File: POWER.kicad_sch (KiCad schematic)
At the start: 42 parts, among them IC1 MP2491CGQB-P, J1 Jack-DC, U1 5V-DCDC, U2 3v3-DCDC, U5 TPS55340RTER

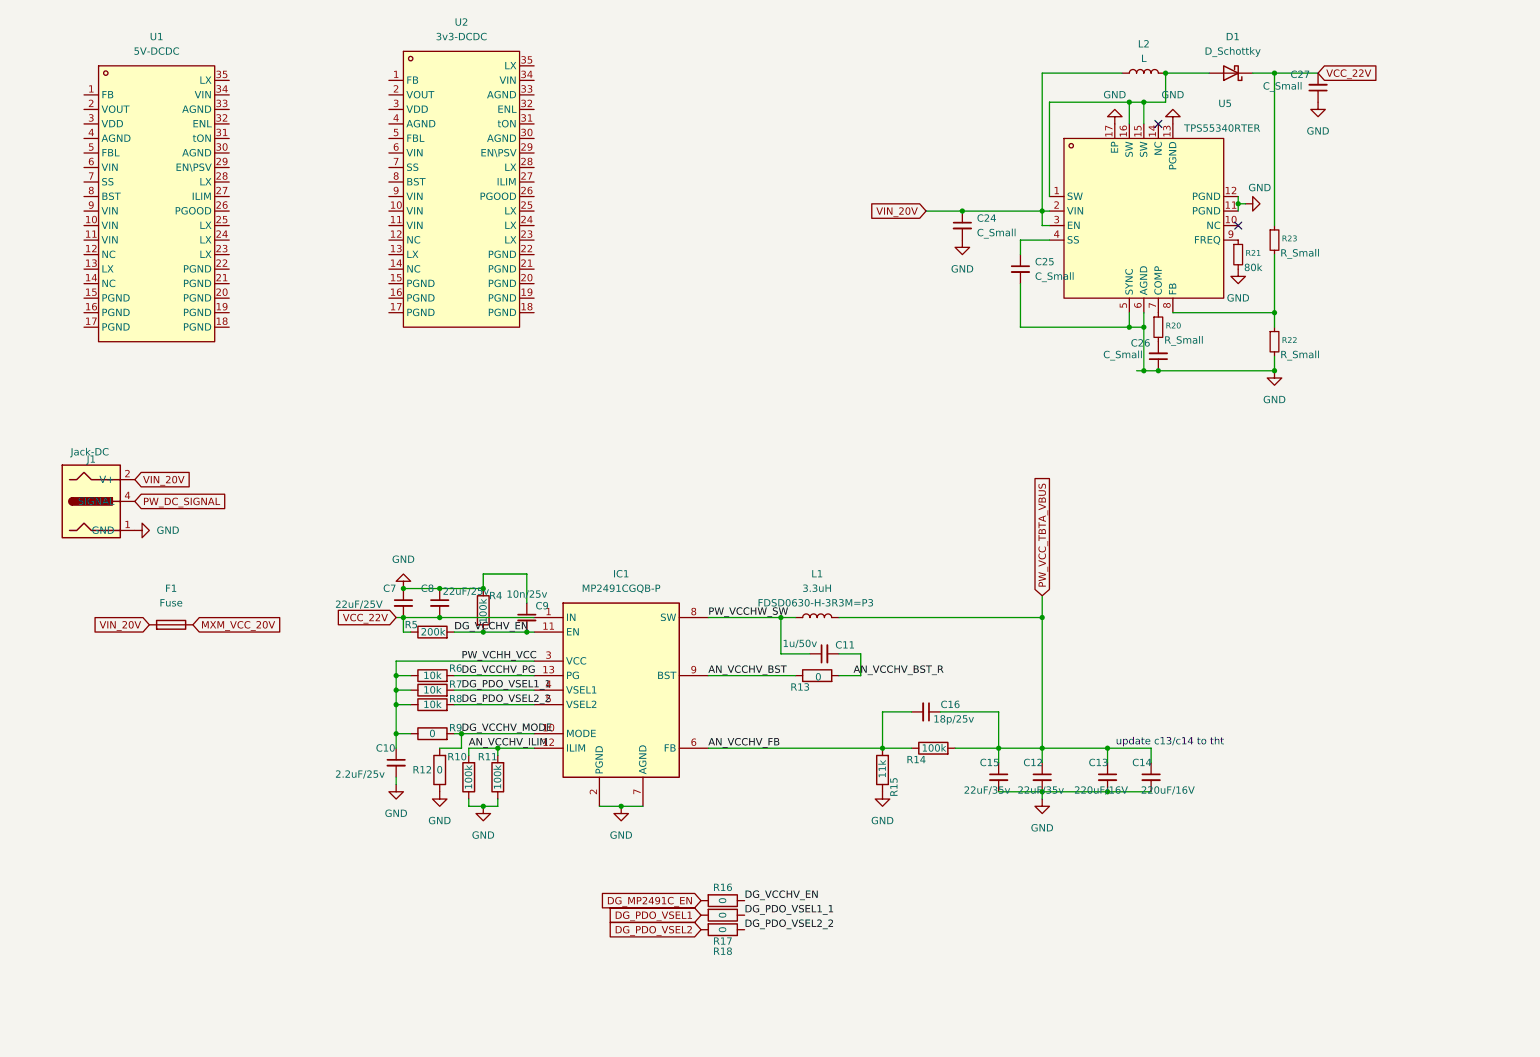
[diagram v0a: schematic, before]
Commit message: update readme.md
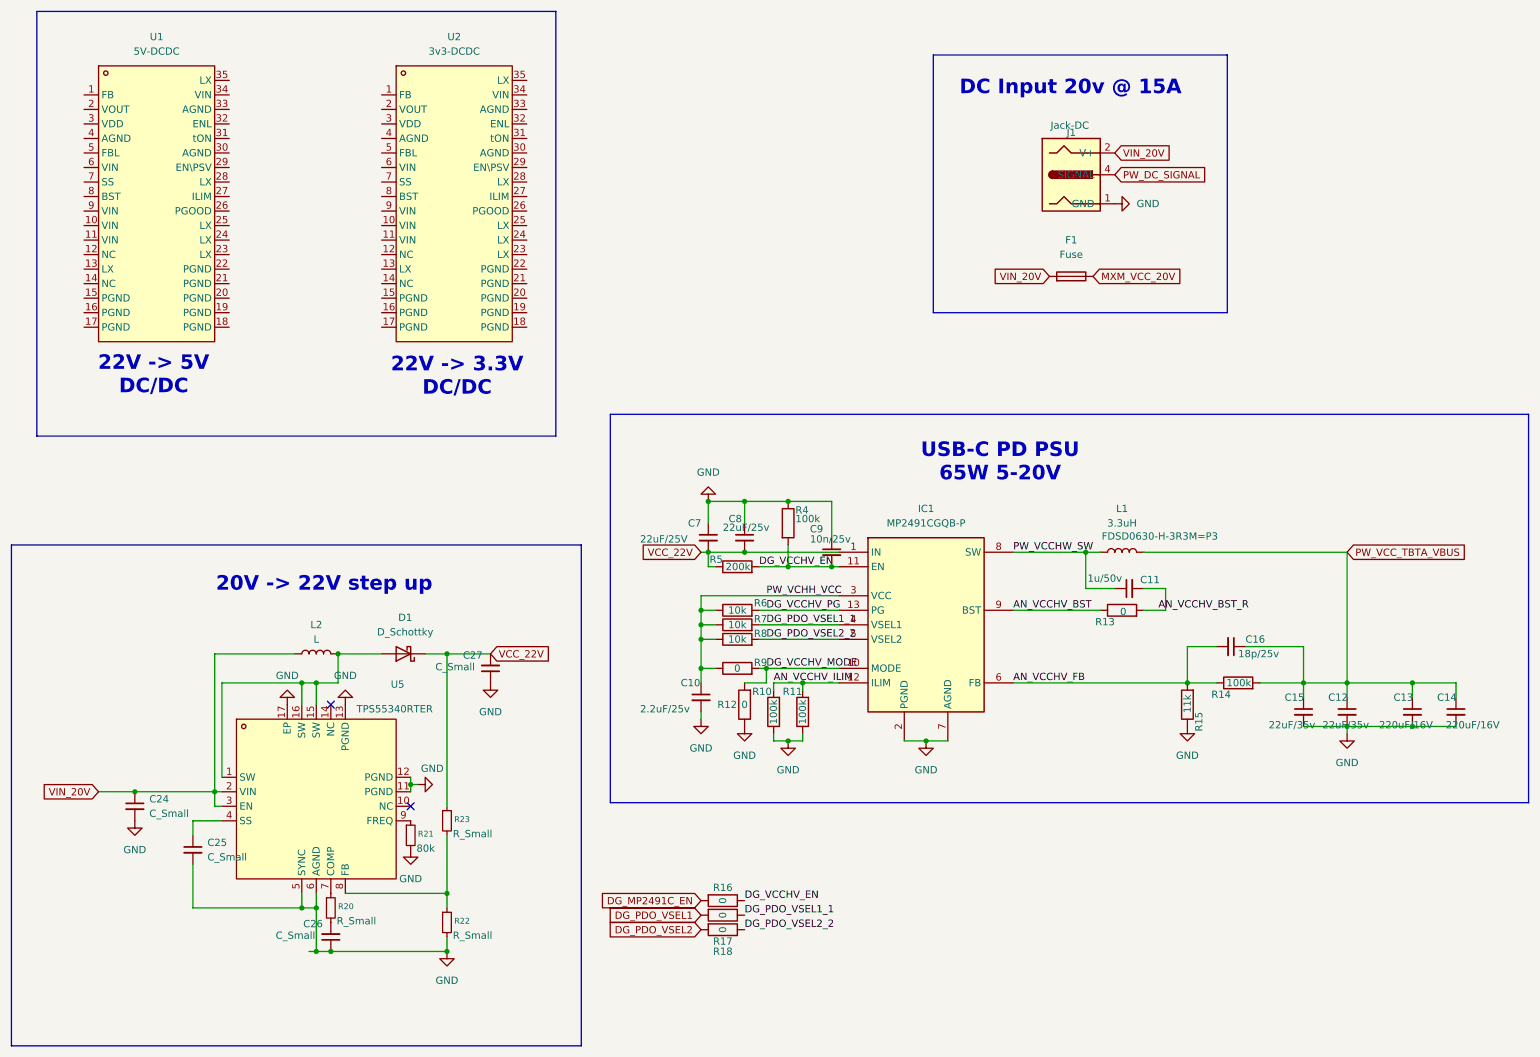
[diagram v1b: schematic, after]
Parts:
- C13, C14: footprint Capacitor_SMD:C_0402_1005Metric -> Capacitor_Tantalum_SMD:CP_EIA-7361-38_AVX-V
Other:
- note added: "20V -> 22V step up"
- note added: "22V -> 3.3V DC/DC"
- note added: "22V -> 5V DC/DC"
- note added: "DC Input 20v @ 15A"
- note added: "USB-C PD PSU 65W 5-20V"
- note removed: "update c13/c14 to tht"
- company: (none) -> mothenjoyer69
- title: (none) -> ThunderMXM
- moved on the sheet: C10, C11, C12, C13, C14, C15, C16, C24, C25, C26, C27, C7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
